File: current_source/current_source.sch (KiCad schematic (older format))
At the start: 14 parts, among them IC1 КР504НТ4, J1 Sensor_R_0-500ohms, U1 MC78L08ACP

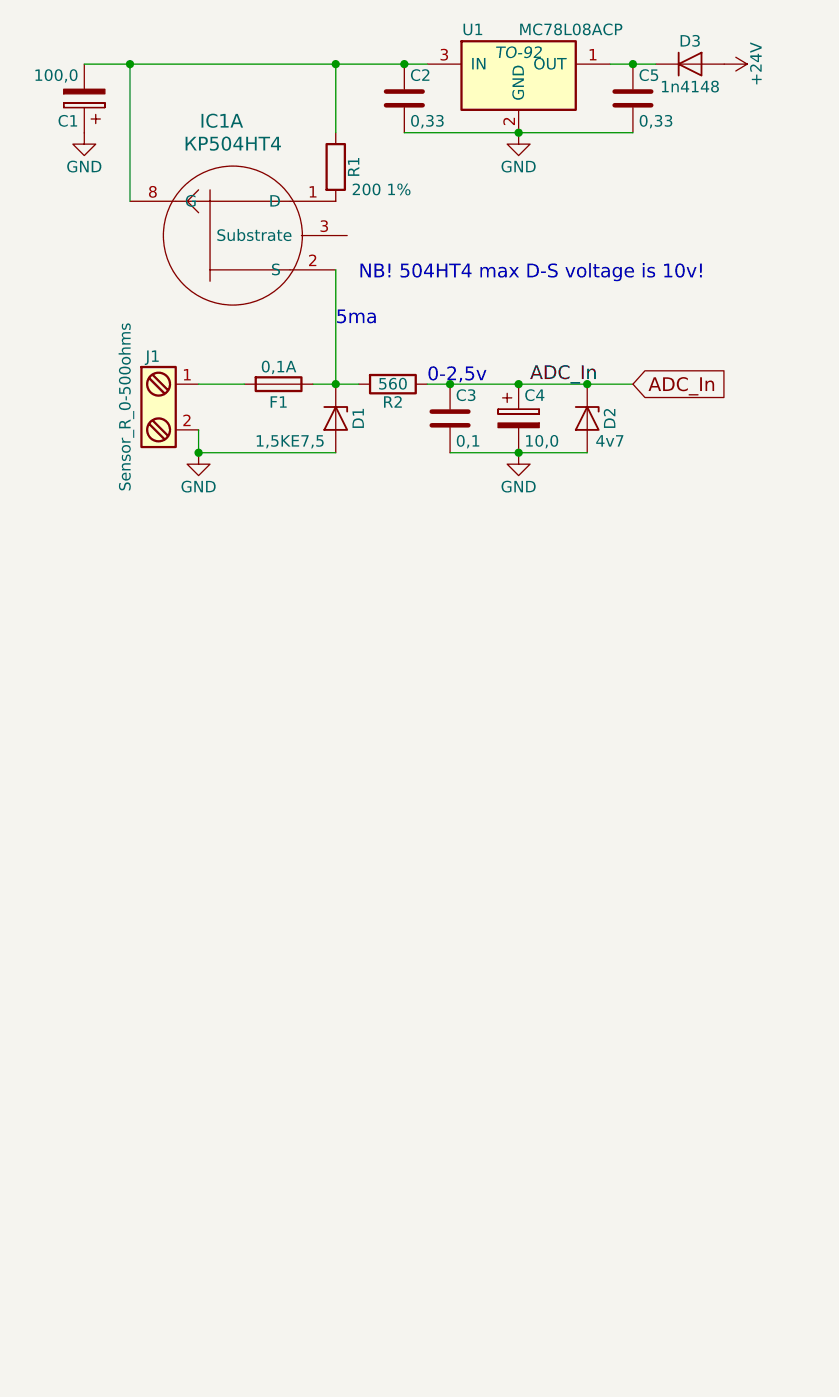
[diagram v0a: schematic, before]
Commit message: template
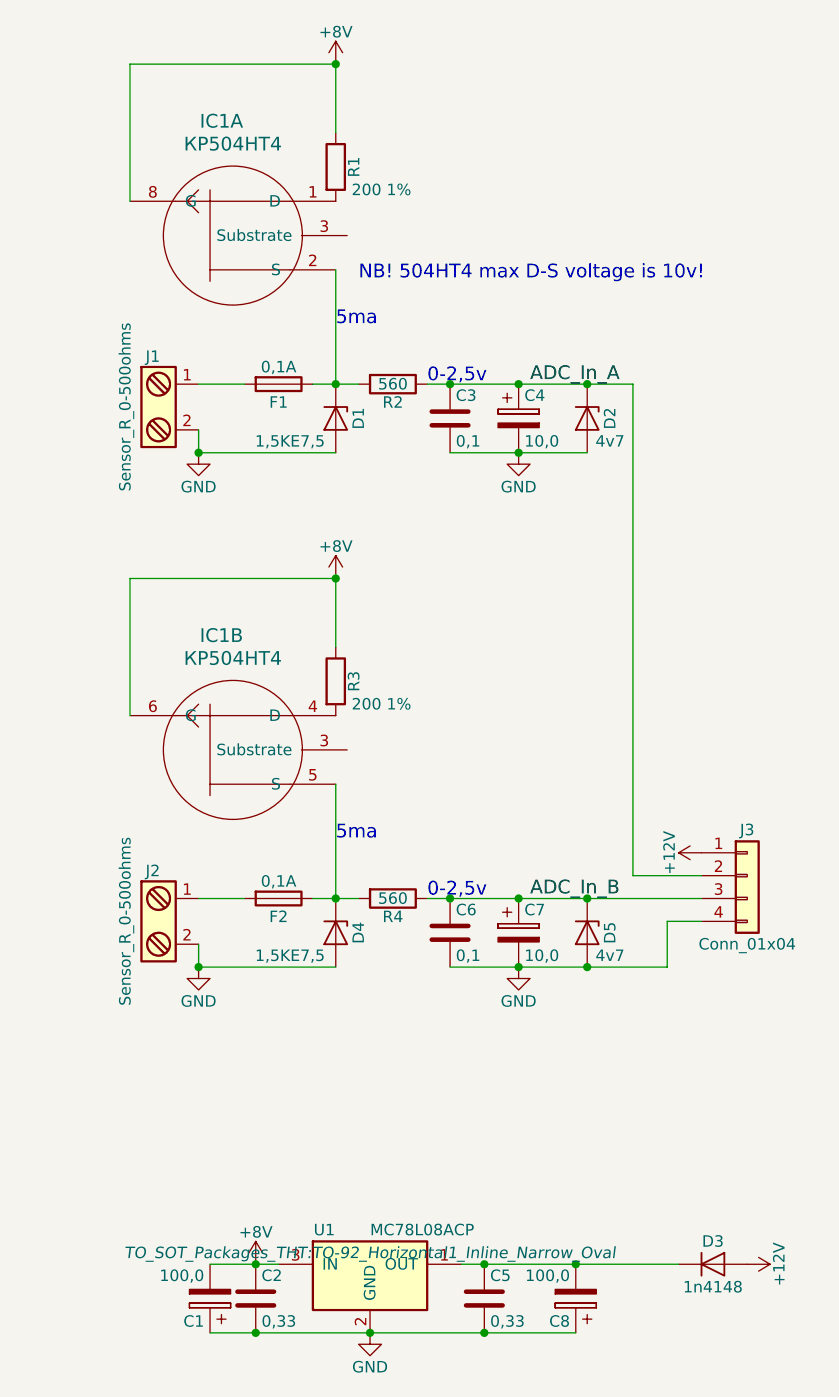
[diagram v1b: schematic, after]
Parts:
- added C6: 0,1, Capacitors_SMD:C_1206_HandSoldering, symbol C
- added C7: 10,0, Capacitors_SMD:CP_Elec_4x5.7, symbol CP
- added C8: 100,0, Capacitors_SMD:CP_Elec_6.3x5.3, symbol CP
- added D4: 1,5KE7,5, Diodes_THT:D_DO-201_P5.08mm_Vertical_AnodeUp, symbol D_Zener
- added D5: 4v7, Diodes_SMD:D_1206, symbol D_Zener
- added F2: 0,1A, Fuse_Holders_and_Fuses:Fuseholder5x20_horiz_open_inline_Type-I, symbol Fuse
- added unit 2 of IC1
- added J2: Sensor_R_0-500ohms, Connectors_Terminal_Blocks:TerminalBlock_bornier-2_P5.08mm, symbol Screw_Terminal_1x02
- added J3: Conn_01x04, Pin_Headers:Pin_Header_Straight_1x04_Pitch2.54mm, symbol Conn_01x04
- added R3: 200 1%, Resistors_THT:R_Axial_DIN0204_L3.6mm_D1.6mm_P2.54mm_Vertical, symbol R
- added R4: 560, Resistors_SMD:R_1206_HandSoldering, symbol R
- C1: footprint (none) -> Capacitors_SMD:CP_Elec_6.3x5.3
- C2, C3, C5: footprint (none) -> Capacitors_SMD:C_1206_HandSoldering
- C4: footprint (none) -> Capacitors_SMD:CP_Elec_4x5.7
- D1: footprint (none) -> Diodes_THT:D_DO-201_P5.08mm_Vertical_AnodeUp
- D2, D3: footprint (none) -> Diodes_SMD:D_1206
- F1: footprint (none) -> Fuse_Holders_and_Fuses:Fuseholder5x20_horiz_open_inline_Type-I
- IC1: footprint (none) -> Housings_DIP:DIP-8_W7.62mm_LongPads
- J1: footprint (none) -> Connectors_Terminal_Blocks:TerminalBlock_bornier-2_P5.08mm
- R1: footprint (none) -> Resistors_THT:R_Axial_DIN0204_L3.6mm_D1.6mm_P2.54mm_Vertical
- R2: footprint (none) -> Resistors_SMD:R_1206_HandSoldering
- U1: footprint TO-92 -> TO_SOT_Packages_THT:TO-92_Horizontal1_Inline_Narrow_Oval
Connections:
- net GND: now also C6.2, C7.2, C8.1, D4.2 (A), D5.2 (A), J2.2, J3.4 (Pin_4)
- net +8V: now reaches C1.2, C2.1, IC1.8 (G), R1.1, U1.3 (IN)
- net +8V: now also IC1.6 (G), R3.1
- net at C5.1, D3.1 (K), U1.1 (OUT): now also C8.2
- net +24V renamed +12V
- net +12V: now also J3.1 (Pin_1)
- net ADC_In renamed ADC_In_A
- net ADC_In_A: now also J3.2 (Pin_2)
- new net: F2.2, J2.1
- new net: D4.1 (K), F2.1, IC1.5 (S), R4.2
- new net: IC1.4 (D), R3.2
- new net ADC_In_B: C6.1, C7.1, D5.1 (K), J3.3 (Pin_3), R4.1
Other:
- moved on the sheet: C1, C2, C5, D3, U1
